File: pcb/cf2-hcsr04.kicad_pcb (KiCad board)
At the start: 2 copper layers, 25.2 x 27.3 mm, 9 parts, among them P1 CF_EXP_LEFT, P2 CF_EXP_RIGHT, U1 DS28E05, U2 REG71050, U3 HC-SR04

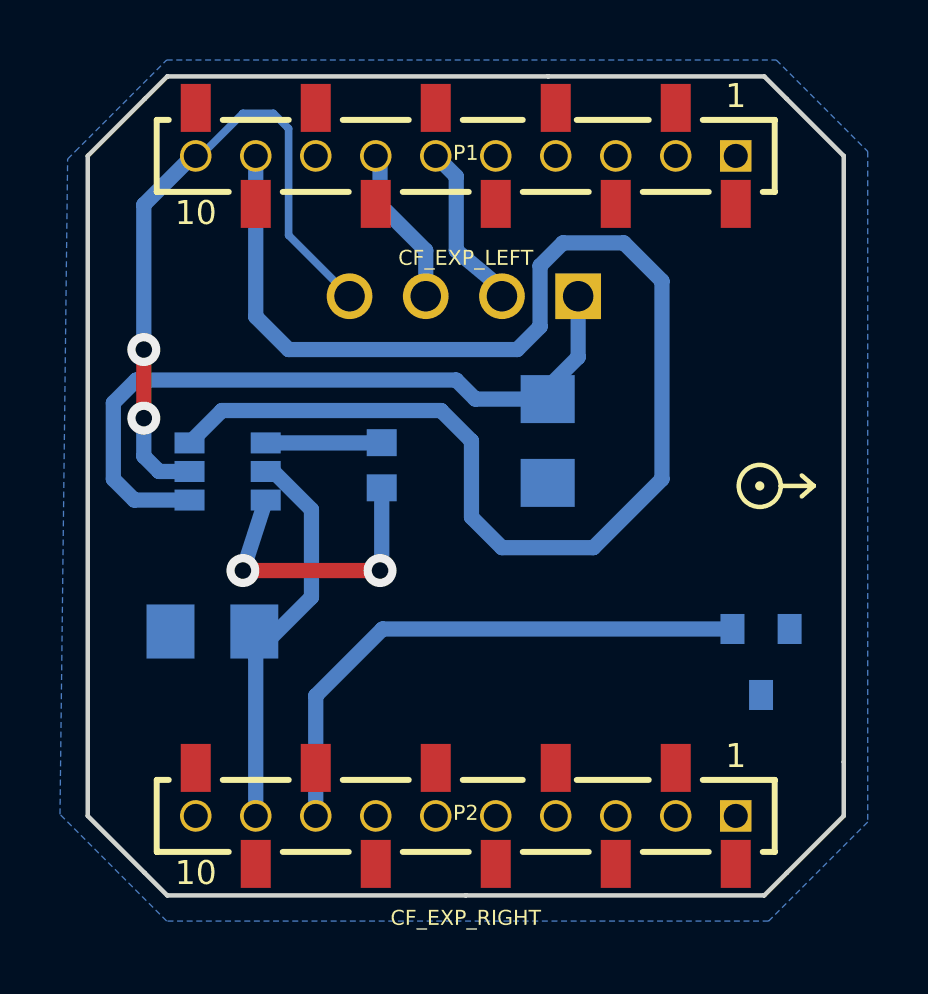
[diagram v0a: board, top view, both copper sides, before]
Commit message: First pcb draft
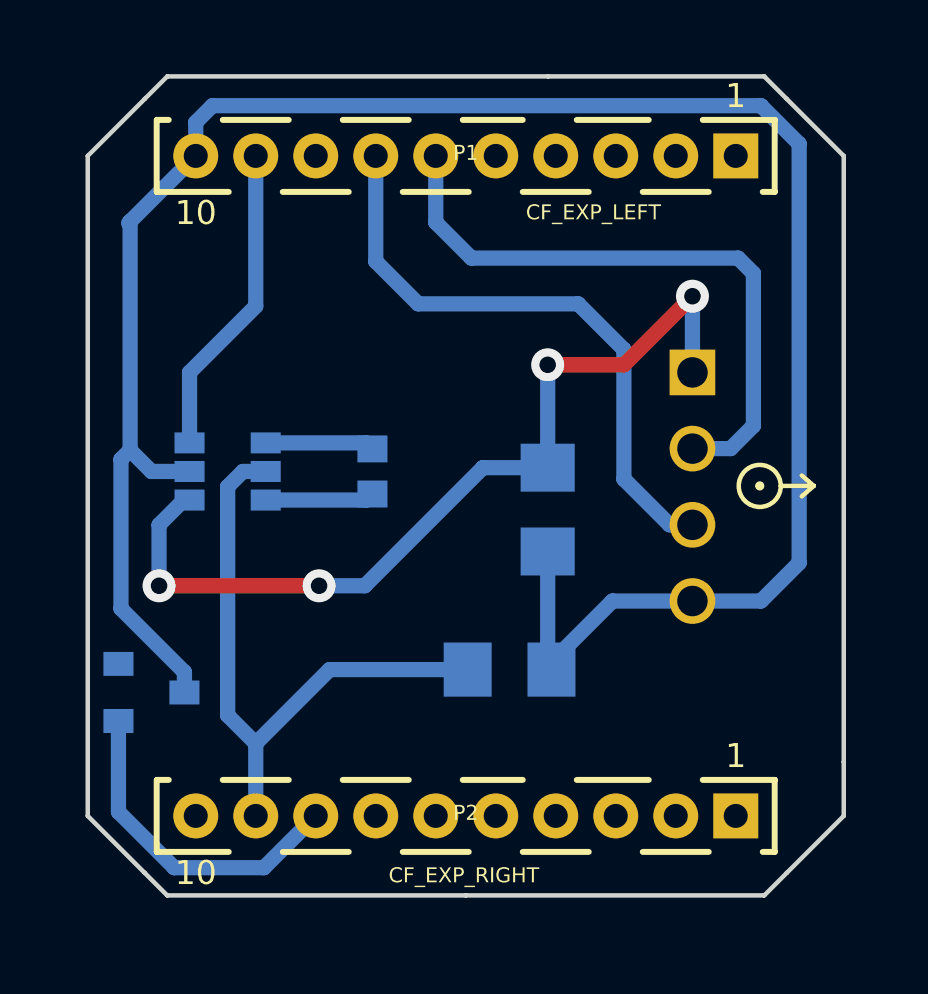
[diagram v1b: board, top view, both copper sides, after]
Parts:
- P1: footprint connectors:BF090-10-X-B2 -> connectors:BF090-10-X-B2-LEFT-NOPADS
- P2: footprint connectors:BF090-10-X-B2 -> connectors:BF090-10-X-B2-RIGHT-NOPADS
- moved U1 20.3 mm to (128.5, 103.9), turned to 90 degrees
- moved C2 9.99 mm to (140.5, 103.1), turned to 0 degrees
- moved U3 9.92 mm to (146.6, 97.0), turned to 270 degrees
- moved C1 2.29 mm to (141.7, 97.8)
- moved C3 0.37 mm to (135.9, 96.5)
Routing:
- net GND: track 22.8 -> 71.7 mm, vias 2 -> 0
- net /IO_4: track 49.7 -> 10.5 mm
- net /IO_1: track 5.67 -> 20.9 mm
- net /IO_2: track 5.37 -> 20.2 mm
- net /OW: track 18.8 -> 11.1 mm
- net /VCOM: track 13.8 -> 20.9 mm
- net N-0000021: track 9.82 -> 3.64 mm, vias 2 -> 0
- net N-0000022: track 24.3 -> 29.7 mm, vias 0 -> 4
- removed copper zone on B.Cu, net GND
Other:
- net class Default: clearance 0.1524 -> 0.0254; trace_width 0.2032 -> 0.508
- rule trace_clearance: 0.1524 -> 0.0254
- rule trace_min: 0.1524 -> 0.254
